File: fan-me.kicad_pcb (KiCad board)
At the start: 2 copper layers, 50 x 30 mm, 14 parts, among them CON1 BARREL_JACK, J1 FAN2, J2 FAN1, U1 LDFPT-TR

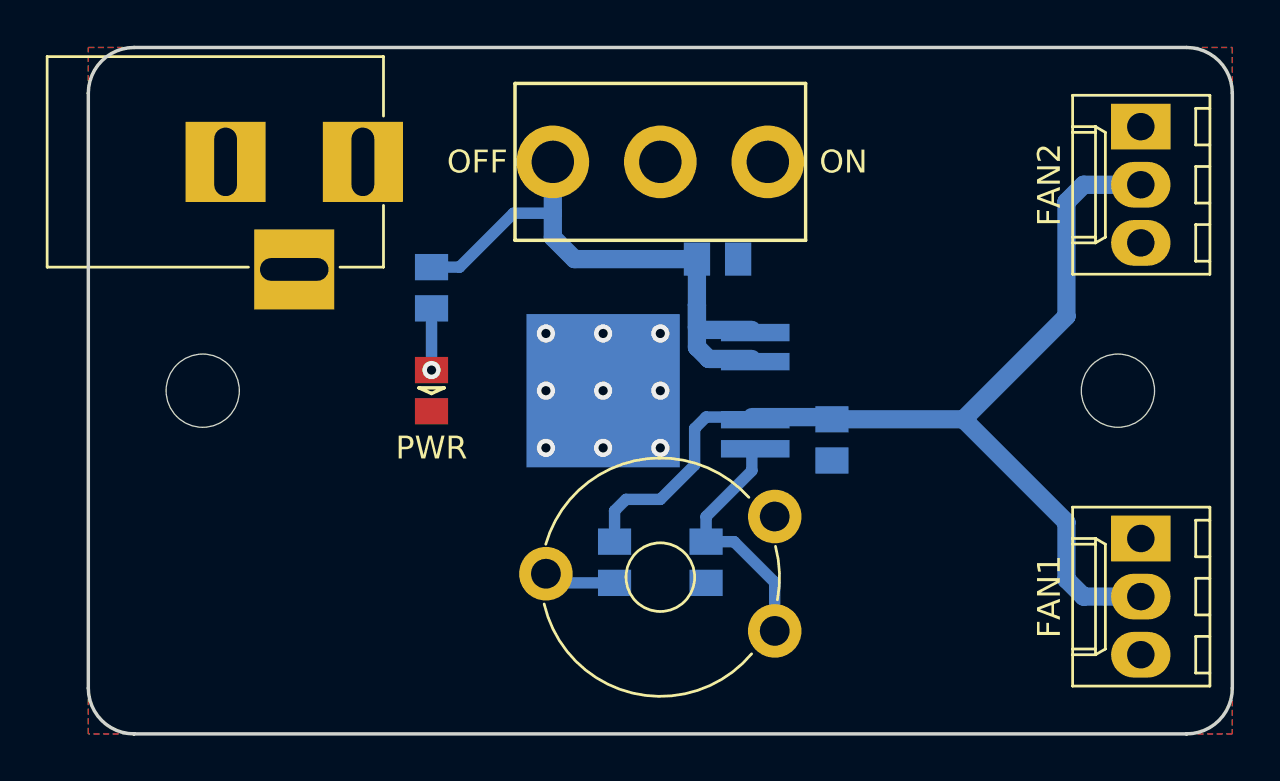
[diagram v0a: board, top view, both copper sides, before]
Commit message: Board smollification mk3
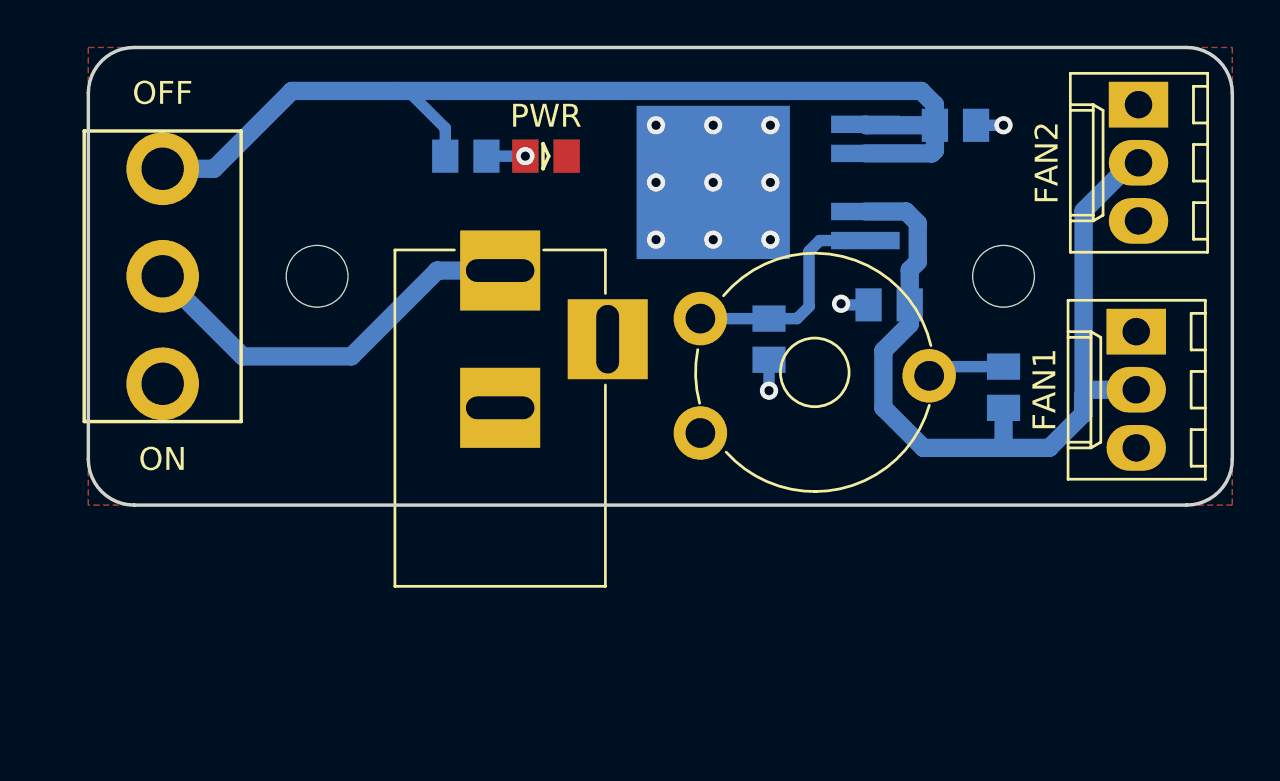
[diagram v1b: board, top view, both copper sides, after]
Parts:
- REF** (x2): footprint Mounting_Holes:MountingHole_3.2mm_M3 -> Mounting_Holes:MountingHole_2.7mm_M2.5
- moved ON 22.3 mm to (53.2, 60.0), turned to 180 degrees
- moved R4 18.6 mm to (90.0, 64.8), turned to 90 degrees
- moved C1 11.9 mm to (87.9, 53.4)
- moved PWR 11.4 mm to (70.0, 54.8), turned to 180 degrees
- moved U1 10.3 mm to (82.5, 55.9)
- moved R3 10.1 mm to (79.8, 62.8)
- moved J2 9.04 mm to (95.8, 62.4)
- moved CON1 7.65 mm to (68.0, 59.8), turned to 90 degrees
- moved REF** 7.07 mm to (90.0, 60.0)
- moved REF** 7.07 mm to (60.0, 60.0)
- moved C2 6.41 mm to (85.0, 61.2), turned to 180 degrees
- moved R1 5.94 mm to (66.5, 54.8), turned to 0 degrees
- moved RV1 4.89 mm to (76.8, 66.8), turned to 0 degrees
- moved J1 0.97 mm to (95.9, 52.5)
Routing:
- net +12V: track 26.2 -> 47.6 mm
- net Net-(CON1-Pad1): track 0.00 -> 17.8 mm
- net Net-(C2-Pad1): track 46.6 -> 38.4 mm
- net GND: track 0.00 -> 3.77 mm, vias 9 -> 12
- net Net-(D1-Pad2): track 2.70 -> 1.70 mm
- net Net-(R3-Pad1): track 10.9 -> 10.0 mm
- removed copper zone on B.Cu, net GND
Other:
- board size 50 x 30 mm -> 50 x 20 mm
